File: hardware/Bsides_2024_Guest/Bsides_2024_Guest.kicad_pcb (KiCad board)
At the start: 2 copper layers, 134.5 x 129.5 mm, 45 parts, among them J1 Add_On, J2 Battery, J3 Battery, J4 OLED, J5 Conn_01x05, J6 Conn_01x05, P1 USB_C_Plug_USB2.0, Q1 DMG3415U-7, SW1 ON, SW2 RESET, SW3 BOOT, SW4 RESET, SW6 RESET, U1 ESP32-C6-WROOM-1U-N4, U2 AP2112K-3.3

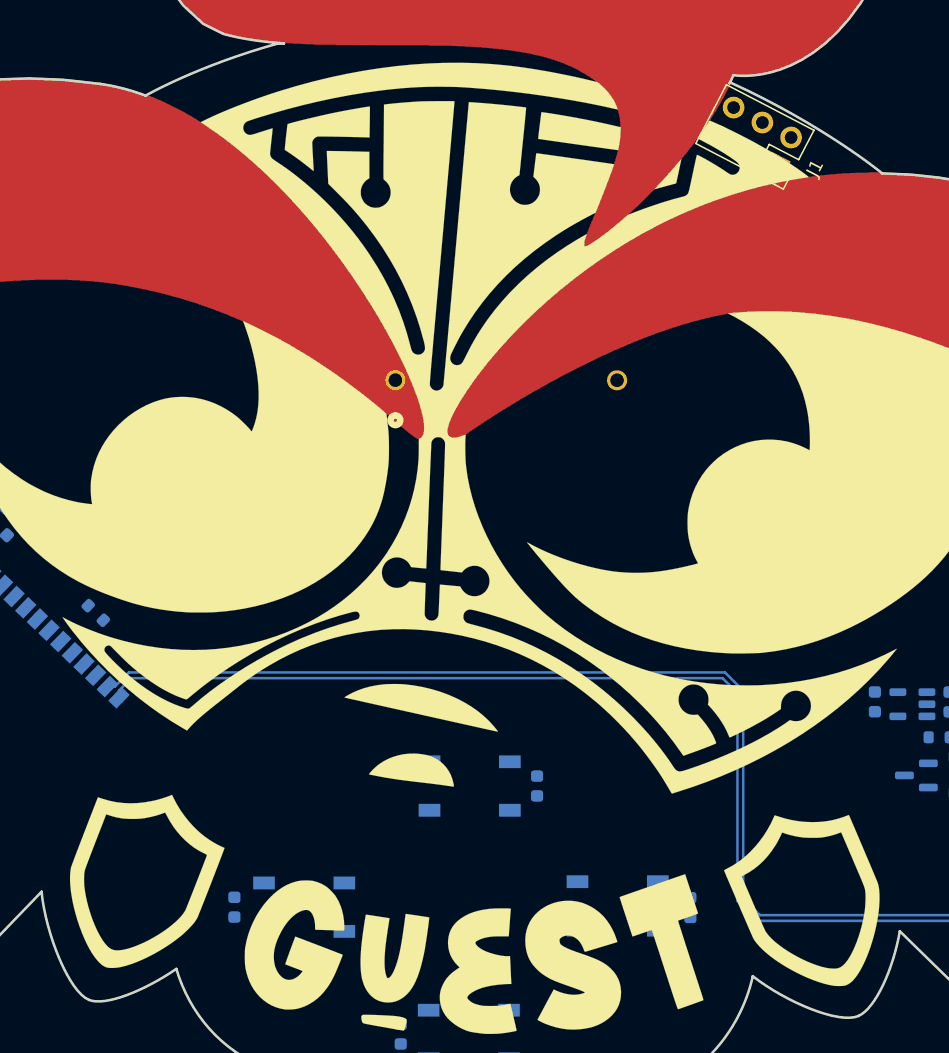
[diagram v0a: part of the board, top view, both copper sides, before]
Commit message: feat(Hw): Update PCB
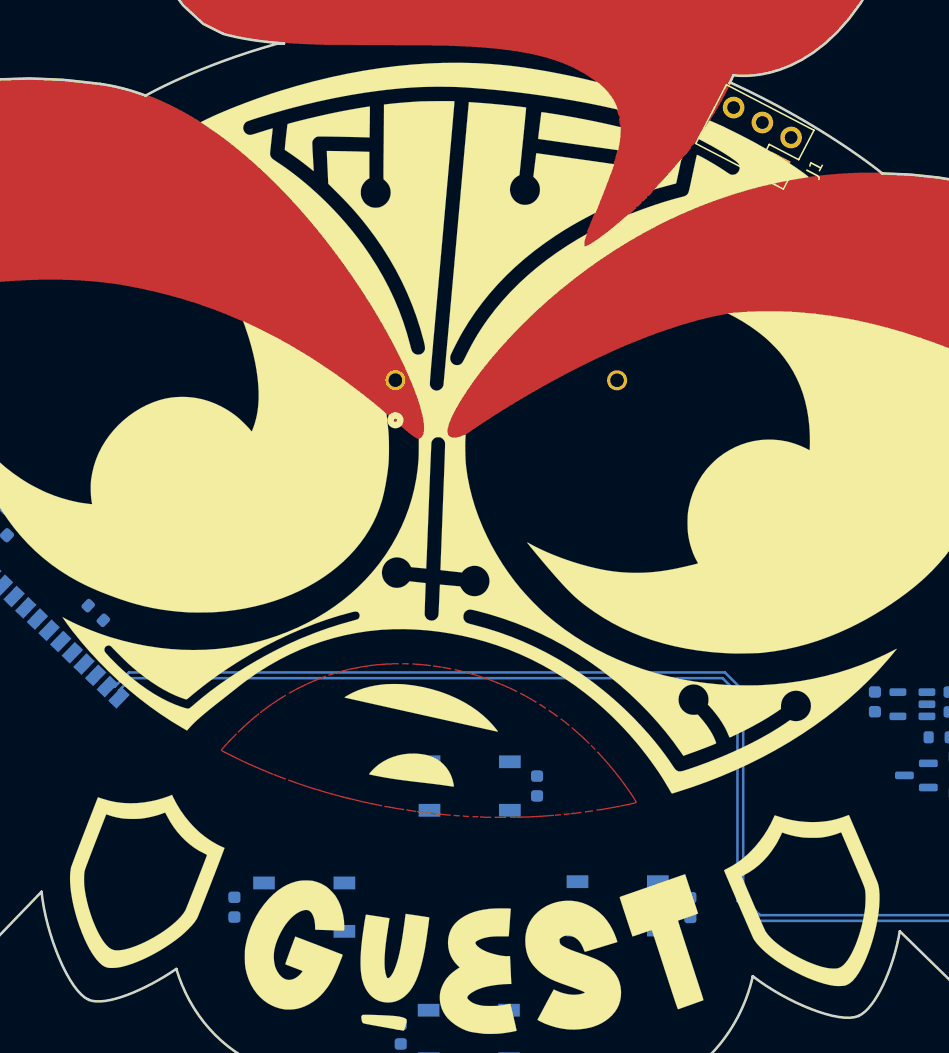
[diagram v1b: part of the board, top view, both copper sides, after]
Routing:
- added copper zone on F.Cu, net (none)
